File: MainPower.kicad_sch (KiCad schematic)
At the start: 73 parts, among them Q3 MBT2222ADW1T1, Q4 MBT2222ADW1T1, U10 ADM1176-1ARMZ-R7, U5 TPS259621DDA, U6 TPS54226PWPR, U7 ADM1176-1ARMZ-R7, U8 TPS259621DDA, U9 TPS54226PWPR

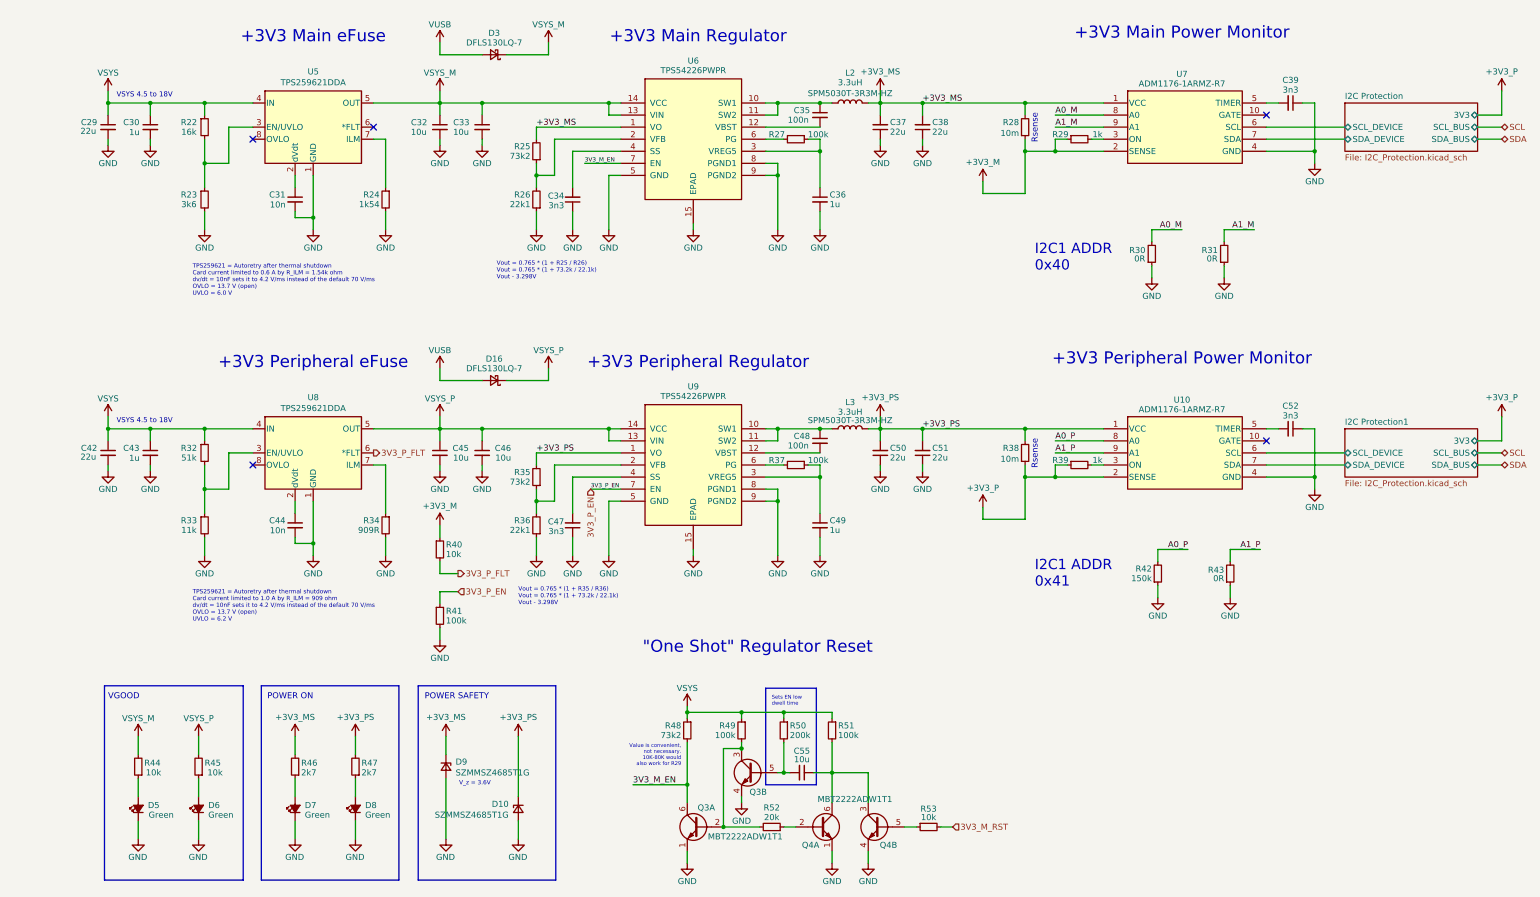
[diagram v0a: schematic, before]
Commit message: v5.0 Updates
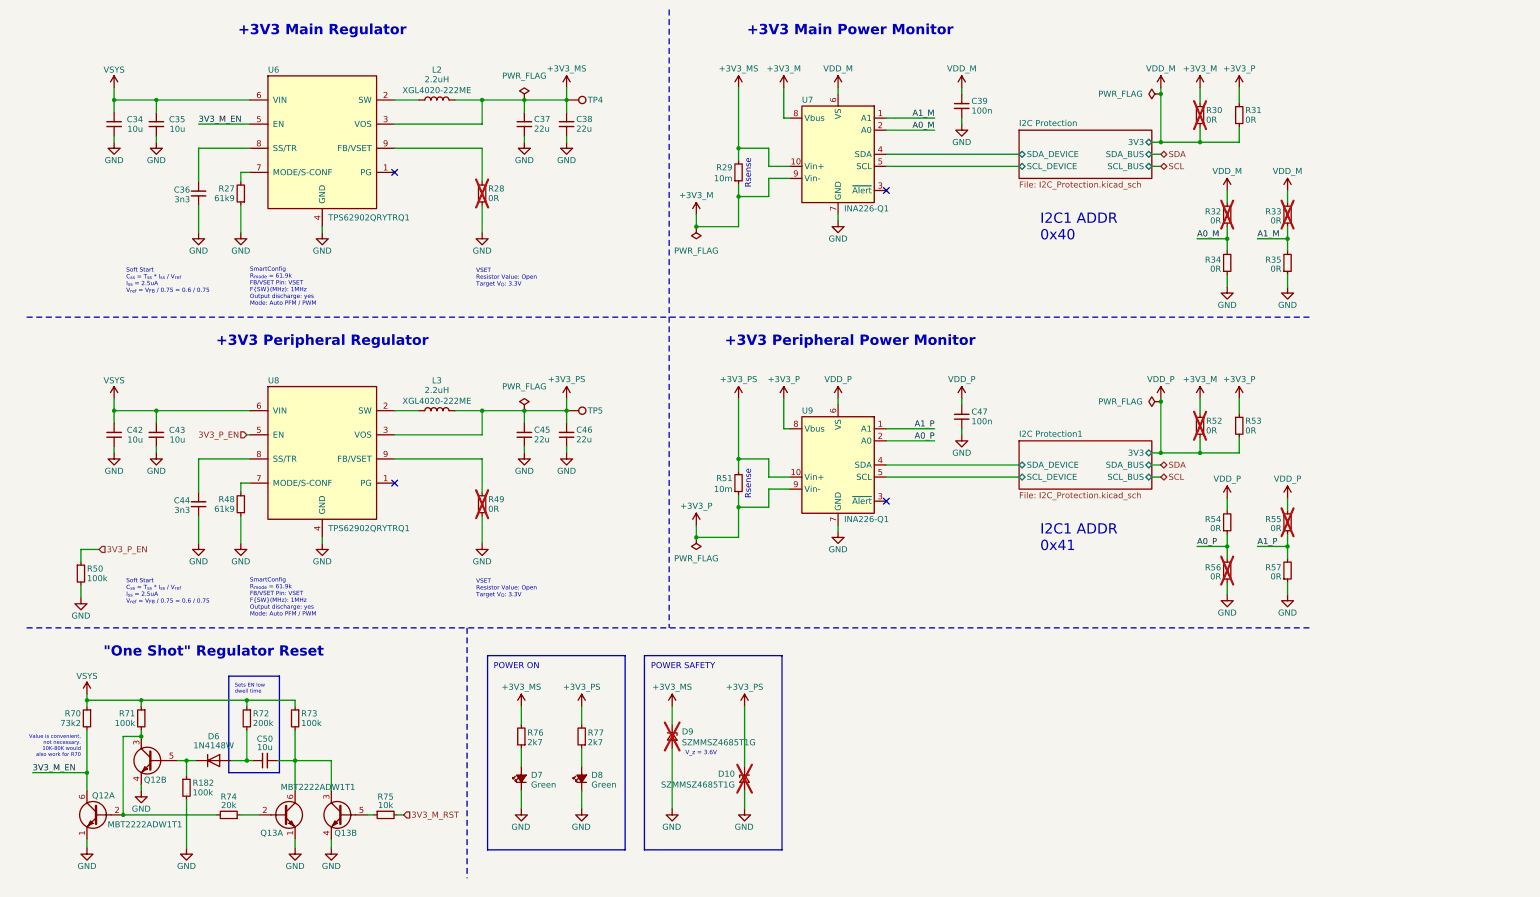
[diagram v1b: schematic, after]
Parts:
- removed C29, C50, C51: 22u, Capacitor_SMD:C_1210_3225Metric, symbol Device:C_Small
- removed C30, C49: 1u, Capacitor_SMD:C_0603_1608Metric, symbol Device:C_Small
- removed C31: 10n, Capacitor_SMD:C_0603_1608Metric, symbol Device:C_Small
- removed C32, C33: 10u, Capacitor_SMD:C_0805_2012Metric, symbol Device:C_Small
- removed C48: 100n, Capacitor_SMD:C_0603_1608Metric, symbol Device:C_Small
- removed C52: 3n3, Capacitor_SMD:C_0603_1608Metric, symbol Device:C_Small
- removed D16, D3: DFLS130LQ-7, Diode_SMD:D_PowerDI-123, symbol Device:D_Schottky_Small
- removed D5, D6: LED_G_0603_LTST-C190GKT, LED_SMD:LED_0603_1608Metric, symbol Device:LED_Small_Filled
- removed R22: 16k, Resistor_SMD:R_0603_1608Metric, symbol Device:R_Small
- removed R23: 3k6, Resistor_SMD:R_0603_1608Metric, symbol Device:R_Small
- removed R24: 1k54, Resistor_SMD:R_0603_1608Metric, symbol Device:R_Small
- removed R25, R35: 73k2, Resistor_SMD:R_0603_1608Metric, symbol Device:R_Small
- removed R26, R36: 22k1, Resistor_SMD:R_0603_1608Metric, symbol Device:R_Small
- removed R34: 909R, Resistor_SMD:R_0603_1608Metric, symbol Device:R_Small
- removed R37: 100k, Resistor_SMD:R_0603_1608Metric, symbol Device:R_Small
- removed R38: 10m, Resistor_SMD:R_2512_6332Metric, symbol Device:R_Small
- removed R39: 1k, Resistor_SMD:R_0603_1608Metric, symbol Device:R_Small
- removed R40, R44, R45: 10k, Resistor_SMD:R_0603_1608Metric, symbol Device:R_Small
- removed R42: 150k, Resistor_SMD:R_0603_1608Metric, symbol Device:R_Small
- removed R43: 0R, Resistor_SMD:R_0603_1608Metric, symbol Device:R_Small
- removed U10, U7: ADM1176-1ARMZ-R7, Package_SO:MSOP-10_3x3mm_P0.5mm, symbol Argus-IC:ADM1176-1ARMZ-R7
- removed U5, U8: TPS259621DDA, Package_SO:Texas_R-PDSO-G8_EP2.95x4.9mm_Mask2.4x3.1mm_ThermalVias, symbol Argus-IC:TPS259621DDA
- removed U6, U9: TPS54226PWPR, Package_SO:TSSOP-14-1EP_4.4x5mm_P0.65mm, symbol Argus-IC:TPS54226PWPR
- added D6: 1N4148W, Diode_SMD:D_SOD-123, symbol Diode:1N4148W
- added R182: 100k, Resistor_SMD:R_0603_1608Metric, symbol Device:R_Small
- added R30, R31, R49, R52, R53, R54, R55, R56, R57: 0R, Resistor_SMD:R_0603_1608Metric, symbol Device:R_Small
- added R48: 61k9, Resistor_SMD:R_0603_1608Metric, symbol Device:R_Small
- added R51: 10m, Resistor_SMD:R_1206_3216Metric, symbol Device:R_Small
- added TP4, TP5: TestPoint, TestPoint:TestPoint_Pad_D1.5mm, symbol Connector:TestPoint
- added U6, U8: TPS62902QRYTRQ1, Argus-IC:TPS62902QRYTRQ1, symbol Argus-IC:TPS62902QRYTRQ1
- added U7, U9: INA226-Q1, Package_SO:TSSOP-10_3x3mm_P0.5mm, symbol Sensor_Energy:INA226
- C34: value 3n3 -> 10u; footprint Capacitor_SMD:C_0603_1608Metric -> Capacitor_SMD:C_0805_2012Metric; MPN C3877267 -> C386084
- C35: value 100n -> 10u; footprint Capacitor_SMD:C_0603_1608Metric -> Capacitor_SMD:C_0805_2012Metric; MPN C307348 -> C386084
- C36: value 1u -> 3n3; MPN C2214844 -> C3877267
- C39, C47: value 3n3 -> 100n; MPN C3877267 -> C2803395
- C42: value 22u -> 10u; footprint Capacitor_SMD:C_1210_3225Metric -> Capacitor_SMD:C_0805_2012Metric; MPN C2803395 -> C386084
- C43: value 1u -> 10u; footprint Capacitor_SMD:C_0603_1608Metric -> Capacitor_SMD:C_0805_2012Metric; MPN C2214844 -> C386084
- C44: value 10n -> 3n3; MPN C161232 -> C3877267
- C45, C46: value 10u -> 22u; footprint Capacitor_SMD:C_0805_2012Metric -> Capacitor_SMD:C_1210_3225Metric; MPN C386084 -> C2803395
- D10, D9: now not fitted; now left out of the parts list
- L2, L3: value 3.3uH -> 2.2uH; footprint Argus-Passives:IND_SPM5030T-3R3M-HZ -> Inductor_SMD:L_Coilcraft_XAL4020-XXX; Field6 SPM5030T-3R3M-HZ -> XGL4020-222ME; MPN C518955 -> (none)
- Q12: renamed from Q3; footprint Package_TO_SOT_SMD:SOT-363_SC-70-6 -> Argus-IC:SOT-363_SC-70-6
- Q13: renamed from Q4; footprint Package_TO_SOT_SMD:SOT-363_SC-70-6 -> Argus-IC:SOT-363_SC-70-6
- R27: value 100k -> 61k9; MPN C237792 -> C844759
- R28: value 10m -> 0R; footprint Resistor_SMD:R_2512_6332Metric -> Resistor_SMD:R_0603_1608Metric; MPN C840621 -> C844759; now not fitted; now left out of the parts list
- R29: value 1k -> 10m; footprint Resistor_SMD:R_0603_1608Metric -> Resistor_SMD:R_1206_3216Metric; MPN C2484712 -> C840621
- R32: value 51k -> 0R; MPN C844796 -> C844915; now not fitted; now left out of the parts list
- R33: value 11k -> 0R; MPN C844734 -> C844915; now not fitted; now left out of the parts list
- renumbered C55 to C50, R30 to R34, R31 to R35, R41 to R50, R48 to R70, R49 to R71, R50 to R72, R51 to R73, R52 to R74, R53 to R75, R46 to R76, R47 to R77
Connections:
- net VSYS_P is gone; now on net GND: C45.1, C46.1
- net +3V3_M: now also R30.1, R52.1, U7.8 (Vbus), U7.9 (Vin-); no longer R28.1
- net +3V3_MS: now also R29.2, TP4.1, U6.3 (VOS), U7.10 (Vin+); no longer R28.2
- net +3V3_P: now also R31.1, R51.1, R53.1, U9.8 (Vbus), U9.9 (Vin-)
- net +3V3_PS: now also C45.2, C46.2, R51.2, TP5.1, U8.3 (VOS), U9.10 (Vin+)
- net 3V3_M_EN: now also U6.5 (EN)
- net 3V3_P_EN: now also U8.5 (EN)
- net A0_M: now also R32.1, U7.2 (A0)
- net A0_P: now also R54.1, R56.2, U9.2 (A0)
- net A1_M: now also R33.1, U7.1 (A1)
- net A1_P: now also R55.1, R57.2, U9.1 (A1)
- net GND: now also C34.2, C35.2, C36.1, C44.1, R27.1, R28.1, R182.2, R48.1, R49.1, R56.1, R57.1, U6.4 (GND), U7.7 (GND), U8.4 (GND), U9.7 (GND); no longer C34.1, C36.2, C44.2, C45.2, C46.2, R33.2
- net I2C Protection/SCL_DEVICE: now also U7.5 (SCL)
- net I2C Protection/SDA_DEVICE: now also U7.4 (SDA)
- net I2C Protection1/SCL_DEVICE: now also U9.5 (SCL)
- net I2C Protection1/SDA_DEVICE: now also U9.4 (SDA)
- net VSYS: now also C34.1, C35.1, U6.6 (VIN), U8.6 (VIN); no longer R32.1
- net VDD_P: now reaches C47.2
- net VDD_P: now also R52.2, R53.2, R54.2, R55.2, U9.6 (VS)
- net VDD_M: now reaches R32.2
- net VDD_M: now also C39.2, R33.2, R30.2, R31.2, U7.6 (VS); no longer R33.1
- net at L2.1: now also U6.2 (SW); no longer C35.1
- net at C50.2, R72.2: now also D6.2 (A); no longer Q12.5 (B2)
- net at L3.1: now also U8.2 (SW)
- net at R27.2: now also U6.7 (MODE/S-CONF)
- new net: D6.1 (K), Q12.5 (B2), R182.1
- new net: R48.2, U8.7 (MODE/S-CONF)
- new net: C44.2, U8.8 (SS/TR)
- new net: R49.2, U8.9 (FB/VSET)
- new net: C36.2, U6.8 (SS/TR)
- new net: R28.2, U6.9 (FB/VSET)
- no-connect marks 5 -> 4
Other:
- note added: "SmartConfig R_{mode} = 61.9k FB/VSET Pin: VSET F{SW}(MHz): 1MHz Output discharge: yes Mode: Auto PFM / PWM"
- note added: "Soft Start C_{ss} = T_{ss} * I_{ss} / V_{ref} I_{ss} = 2.5uA V_{ref} = V_{FB} / 0.75 = 0.6 / 0.75"
- note added: "VSET Resistor Value: Open Target V_{O}: 3.3V"
- note added: "Value is convenient, not necessary. 10K-80K would also work for R70"
- note removed: "+3V3 Main eFuse"
- note removed: "+3V3 Peripheral eFuse"
- note removed: "TPS259621 = Autoretry after thermal shutdown Card current limited to 0.6 A by R_ILM = 1.54k ohm dv/dt = 10nF sets it to 4.2 V/ms instead of the default 70 V/ms OVLO = 13.7 V (open) UVLO = 6.0 V"
- note removed: "TPS259621 = Autoretry after thermal shutdown Card current limited to 1.0 A by R_ILM = 909 ohm dv/dt = 10nF sets it to 4.2 V/ms instead of the default 70 V/ms OVLO = 13.7 V (open) UVLO = 6.2 V"
- note removed: "VGOOD"
- note removed: "VSYS 4.5 to 18V"
- note removed: "Value is convenient, not necessary. 10K-80K would also work for R29"
- note removed: "Vout = 0.765 * (1 + R25 / R26) Vout = 0.765 * (1 + 73.2k / 22.1k) Vout - 3.298V"
- note removed: "Vout = 0.765 * (1 + R35 / R36) Vout = 0.765 * (1 + 73.2k / 22.1k) Vout - 3.298V"
- moved on the sheet: C50, D7, D8, Q12A, Q12B, Q13A, Q13B, R34, R35, R50, R70, R71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
